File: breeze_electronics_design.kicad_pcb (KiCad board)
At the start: 2 copper layers, 104.1 x 104.1 mm, 104 parts, among them J1 SIP4, M1 MotorA, M2 MotorB, M3 MotorA, M4 MotorB, Q1 S8050, Q2 SI2302, Q3 SI2302, Q4 SI2302, Q5 SI2302, U1 MIC5205-3.3, U10 NRF24L01, U11 HM_Bluetooth, U2 STM32F103T8U6TR, U3 LM27313, U4 LTC4054, U5 CP2102, U6 MIC5205, U7 HMC5883L, U8 MPU6050, U9 MS5611, X1 16MHZ, Y1 8MHZ

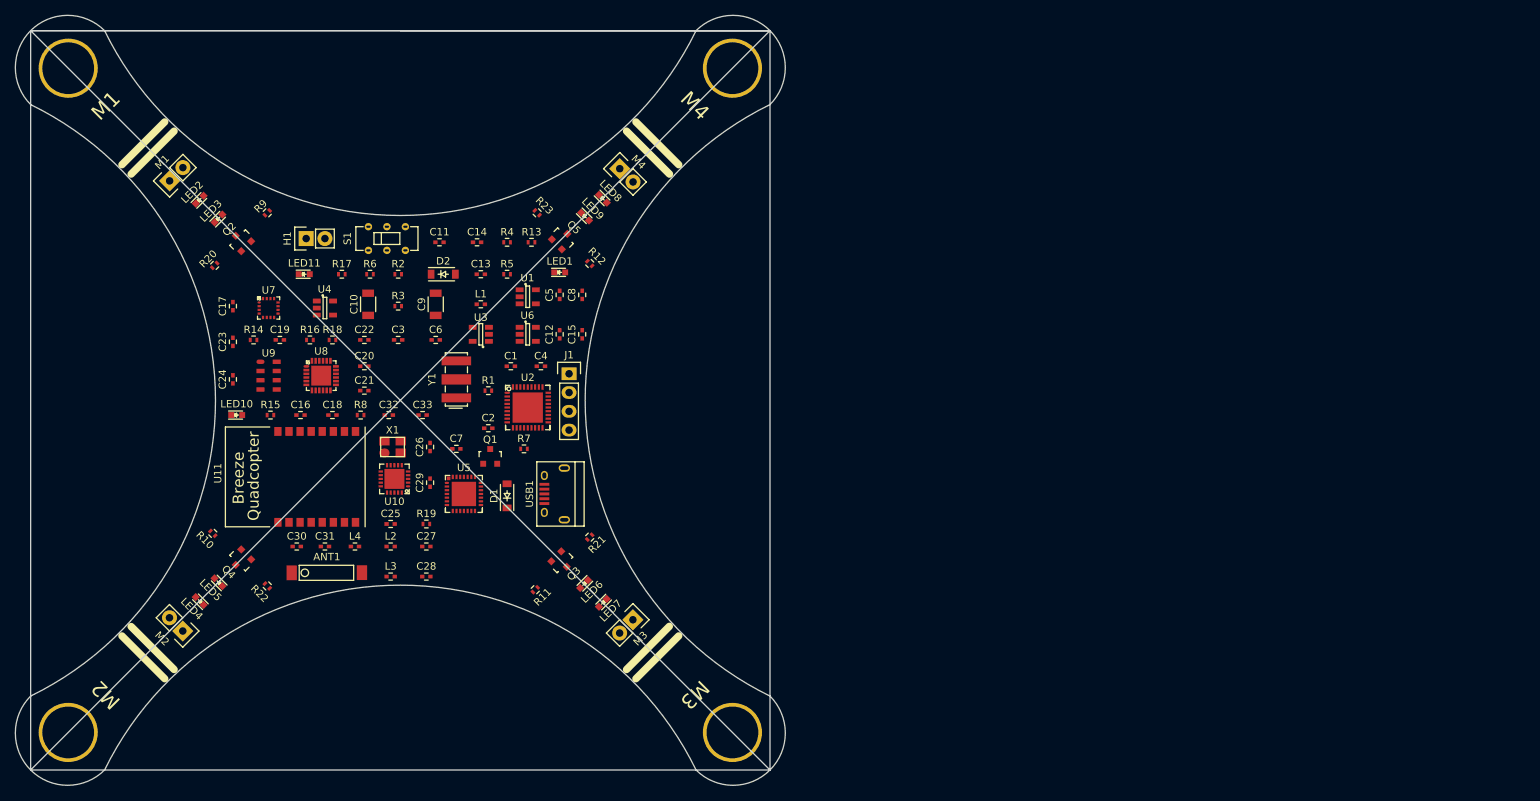
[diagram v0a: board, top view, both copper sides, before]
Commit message: Finish the basic check of layout
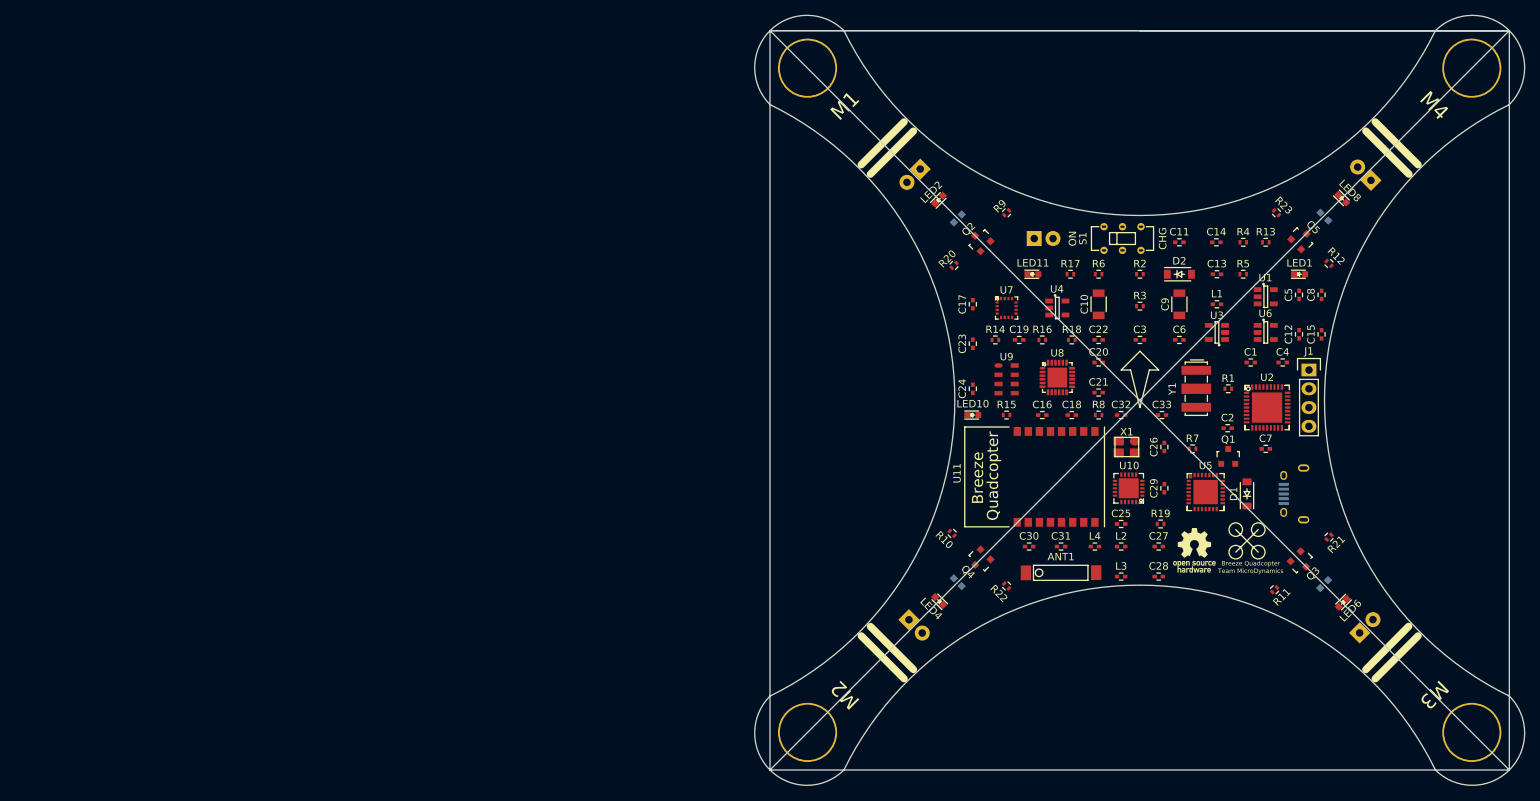
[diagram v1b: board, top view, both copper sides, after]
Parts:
- removed the ? at (-94.9, -94.9)
- removed the ? at (-94.9, -5.08)
- removed the ? at (-5.08, -5.08)
- removed the ? at (-5.08, -94.9)
- added ?: , Footprint:PTH_Motor, F.Cu at (5.08, -94.9)
- added ?: Motor, Footprint:PTH_Motor, F.Cu at (94.9, -5.08)
- added ?: Motor, Footprint:PTH_Motor, F.Cu at (94.9, -94.9)
- added ?: Motor, Footprint:PTH_Motor, F.Cu at (5.08, -5.08)
- added REF**: LOGO_Arrow, Footprint:LOGO_Arrow, F.Cu at (50.0, -54.1)
- added REF**: LOGO_Project, Footprint:LOGO_Project, F.Cu at (64.5, -31.0)
- added REF***: OSHW-Logo_5.7x6mm_SilkScreen, Symbols:OSHW-Logo_5.7x6mm_SilkScreen, F.Cu at (57.4, -29.7)
- H1, LED3, LED5, LED7, LED9, M1, M2, M3, M4, USB1: moved to B.Cu
- S1: footprint Footprint:DIP_SW2x3 -> DIP_SW2x3
- moved C7 109.5 mm to (67.1, -43.4)
- moved LED6 102.6 mm to (77.5, -22.6)
- moved M4 101.6 mm to (81.3, -79.8)
- moved M1 101.5 mm to (20.3, -81.3)
- moved C6 100.6 mm to (55.4, -58.2)
- moved C9 100.6 mm to (55.4, -63.0)
- moved C4 100.3 mm to (69.3, -55.1)
- moved U5 100.3 mm to (58.9, -37.6)
- moved C16 100.3 mm to (36.8, -48.0)
- moved C3 100.3 mm to (50.0, -58.2)
- moved R14 100.3 mm to (30.5, -58.2)
- moved R2 100.3 mm to (50.0, -67.1)
- moved R3 100.3 mm to (50.0, -62.7)
- moved C24 100.1 mm to (27.4, -51.6)
- moved Y1 100.1 mm to (57.7, -51.6), turned to 270 degrees
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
